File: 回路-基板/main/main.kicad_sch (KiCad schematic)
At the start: 55 parts, among them J1 Conn_01x07_Pin, J2 Conn_01x08_Pin, J3 Conn_01x08_Pin, J4 Conn_01x08_Pin, J5 Conn_01x08_Pin, SW1 SW_Push, SW2 SW_Push, SW3 SW_Push, SW4 SW_Push, SW5 SW_Push, SW6 SW_Push, SW7 SW_Push, SW8 SW_SPDT, U1 TWE-L-WX, U2 LM1117MP-3.3

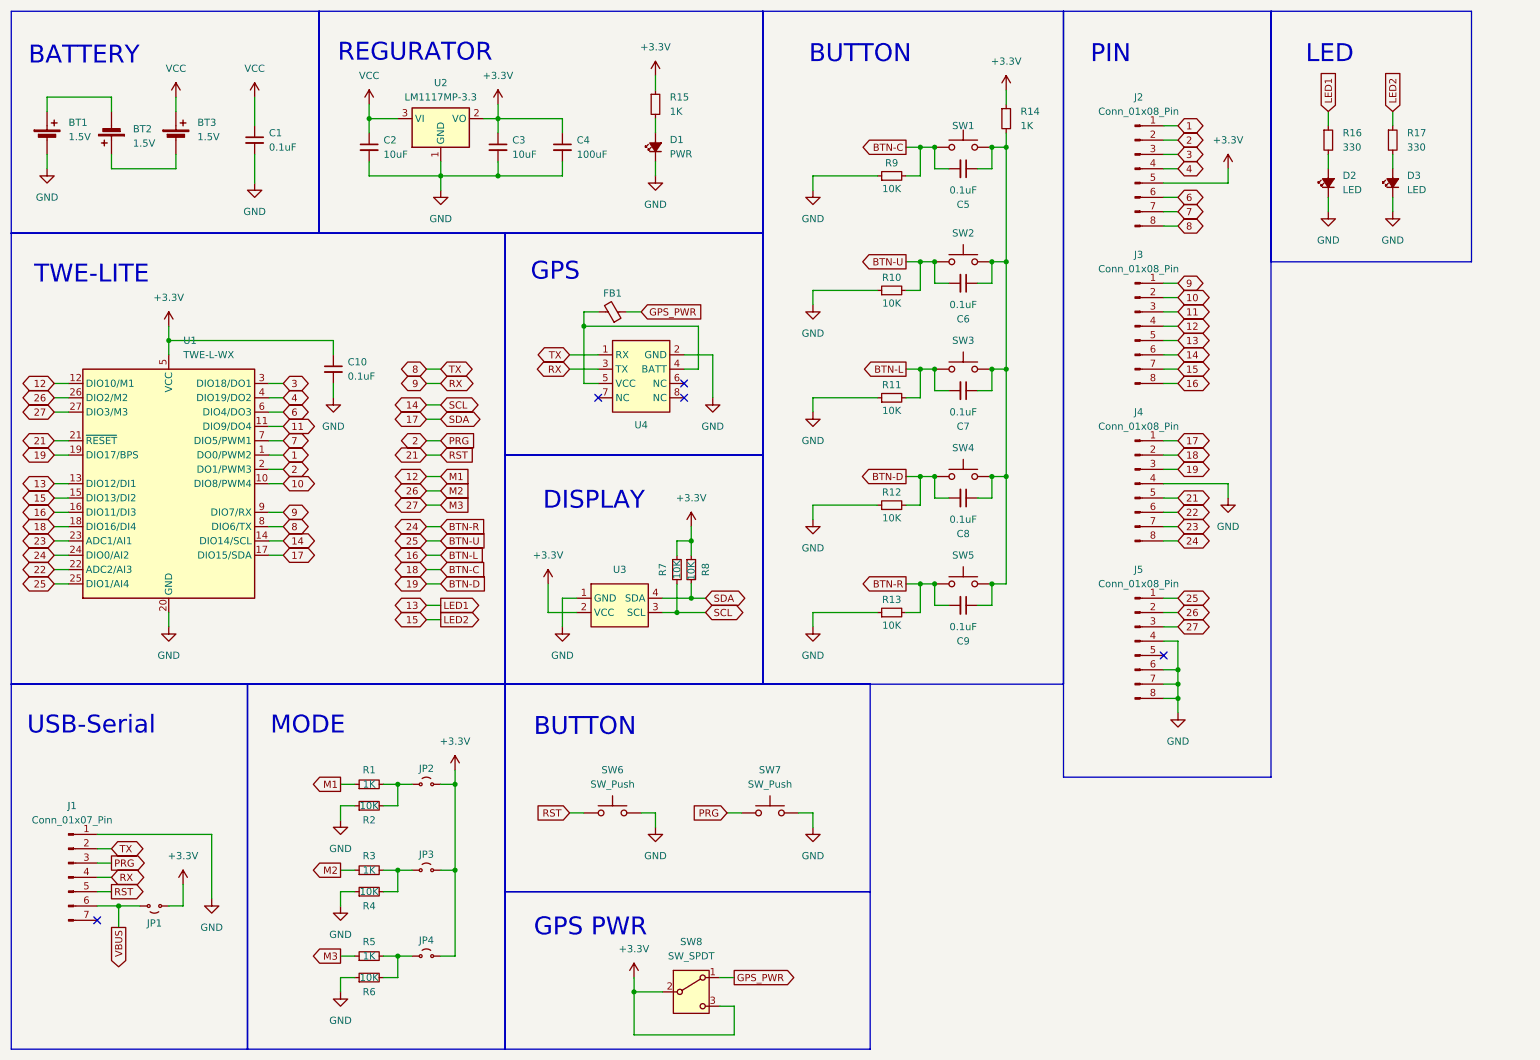
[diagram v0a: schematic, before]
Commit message: 事後プレゼン更新&基板回路図/PCBデザイン更新
DRとかいろいろちぇっくよろしくー
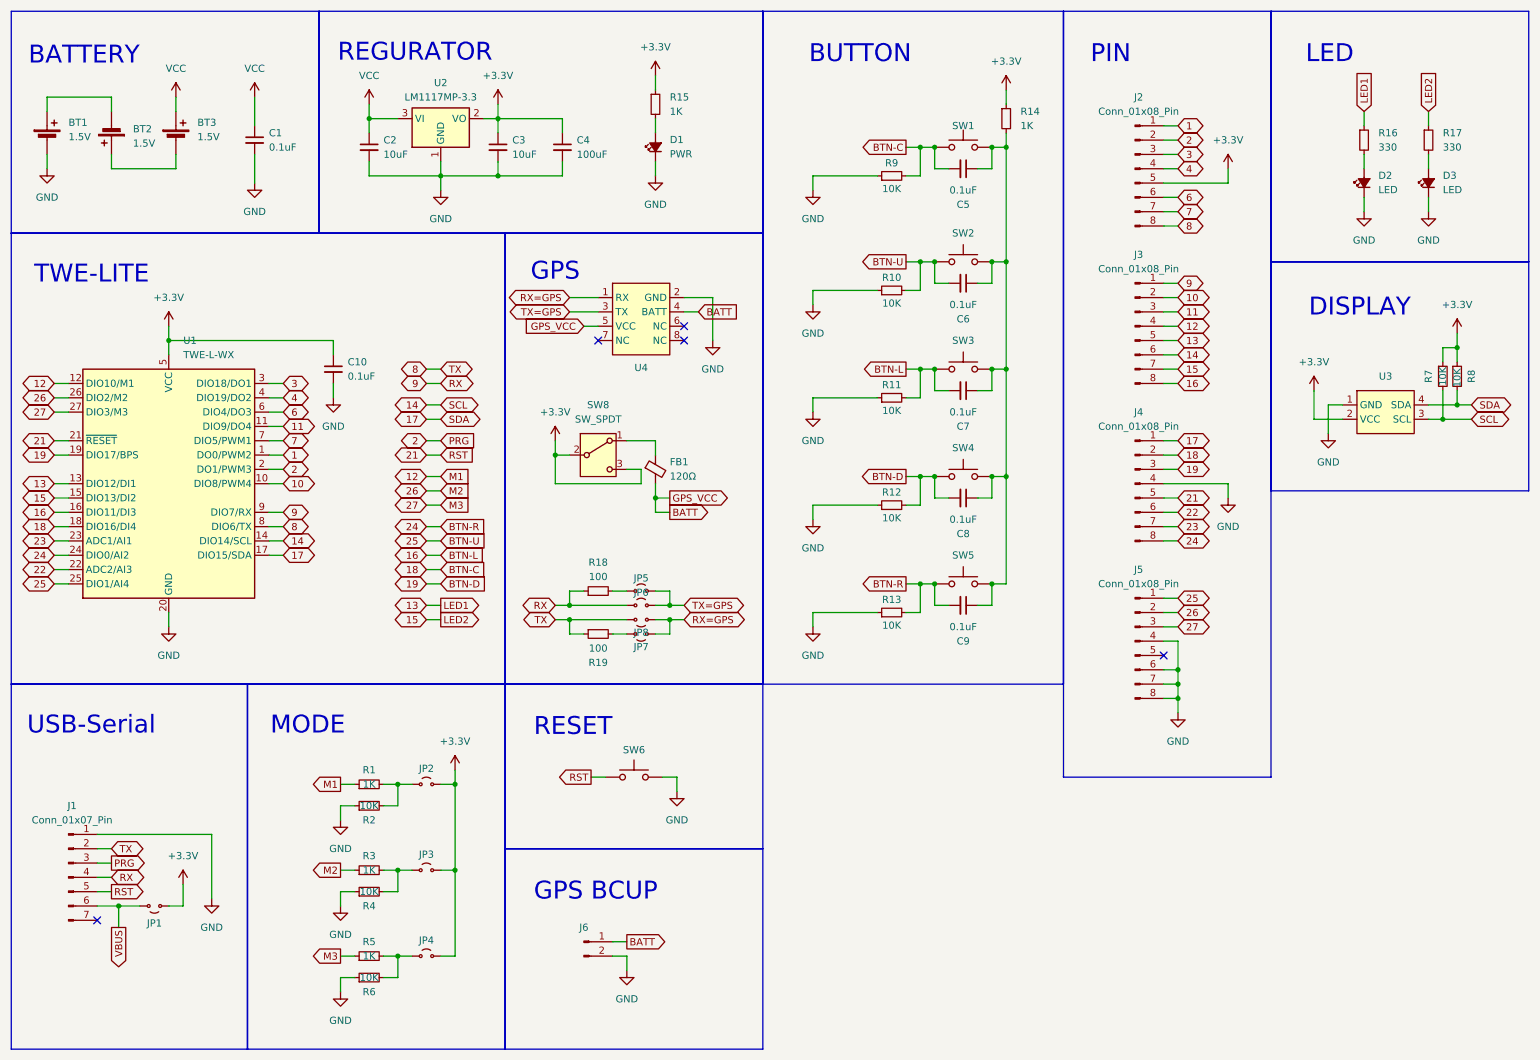
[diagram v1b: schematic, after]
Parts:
- removed SW7: SW_Push, @2024-cansat:Tactile1, symbol Switch:SW_Push
- added J6: Conn_01x02_Pin, Connector_PinSocket_2.54mm:PinSocket_1x02_P2.54mm_Vertical, symbol Connector:Conn_01x02_Pin
- added JP5, JP6, JP7, JP8: Jumper_2_Small_Open, Jumper:SolderJumper-2_P1.3mm_Open_RoundedPad1.0x1.5mm, symbol Jumper:Jumper_2_Small_Open
- added R18, R19: 100, Resistor_SMD:R_0805_2012Metric, symbol Device:R_Small
- FB1: value FerriteBead_Small -> 120Ω
- SW8: footprint @2024-Power:SS12D01G4 -> @2024-cansat:SS12D01G4
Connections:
- net 8: now also JP8.1 (A), R19.1; no longer U4.1 (RX)
- net 9: now also JP6.1 (A), R18.1; no longer U4.3 (TX)
- net GND: now also J6.2 (Pin_2)
- net BATT: now reaches FB1.2, U4.4 (BATT), U4.5 (VCC)
- net BATT: now also J6.1 (Pin_1)
- net GPS_PWR: no longer names the net of FB1.1, SW8.1 (A)
- new net: JP5.1 (A), R18.2
- new net: JP7.1 (A), R19.2
- new net RX=GPS: JP7.2 (B), JP8.2 (B), U4.1 (RX)
- new net TX=GPS: JP5.2 (B), JP6.2 (B), U4.3 (TX)
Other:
- note added: "GPS BCUP"
- note added: "RESET"
- note removed: "GPS PWR"
- moved on the sheet: D2, D3, R16, R17, R7, R8, SW6, SW8, U3, U4
